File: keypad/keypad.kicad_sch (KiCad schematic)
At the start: 7 parts, among them U1 STM32G031G8Ux

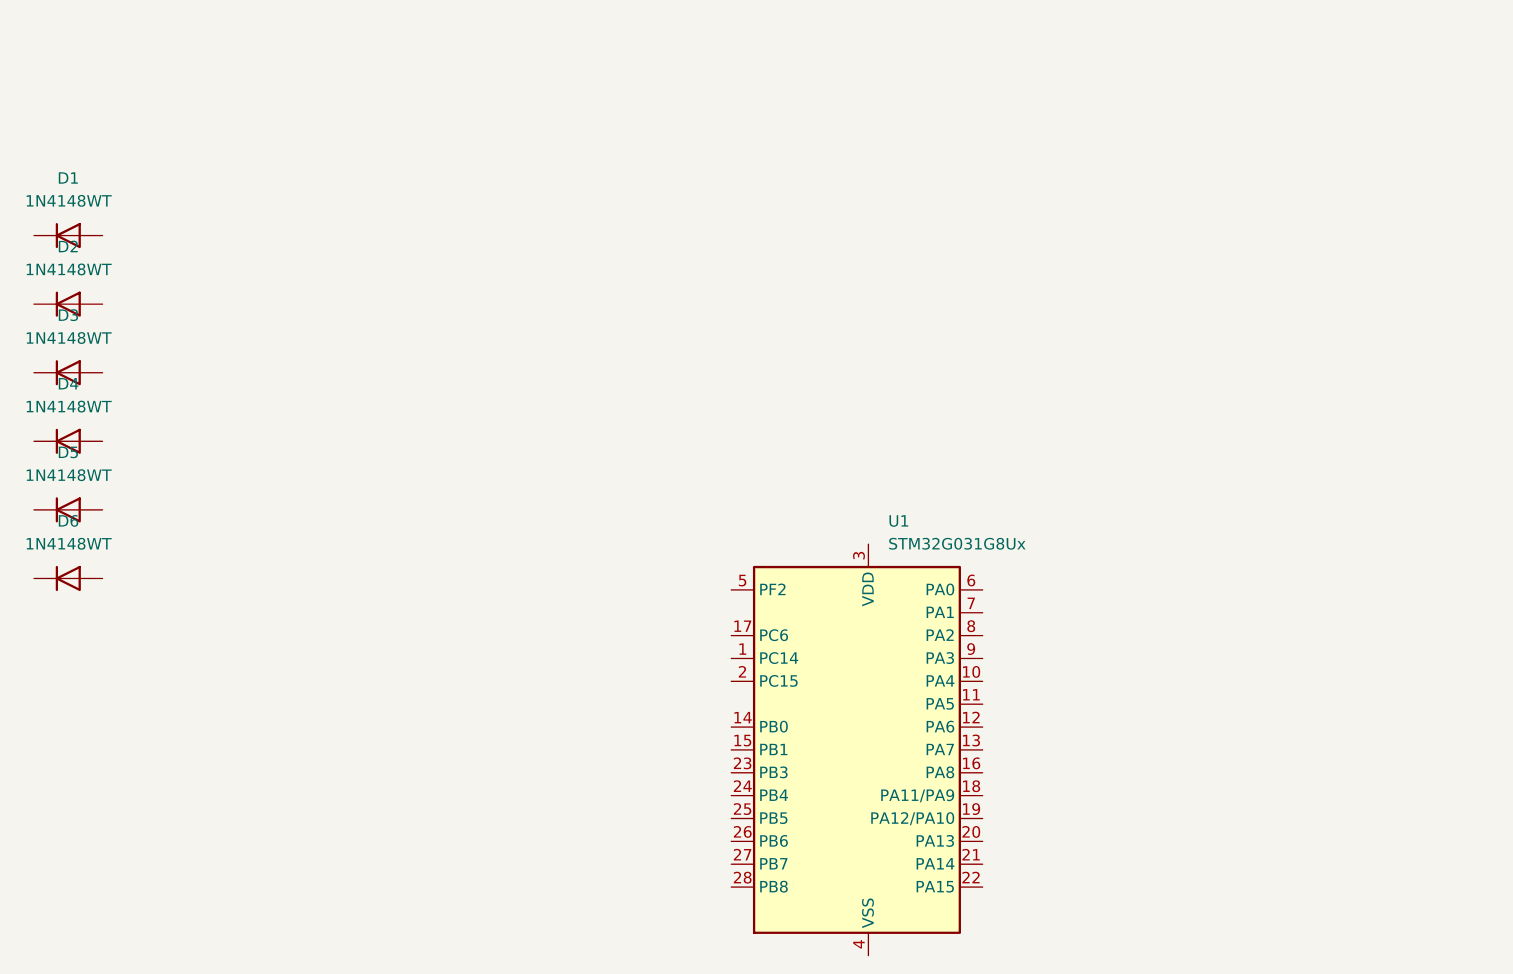
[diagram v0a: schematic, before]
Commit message: main
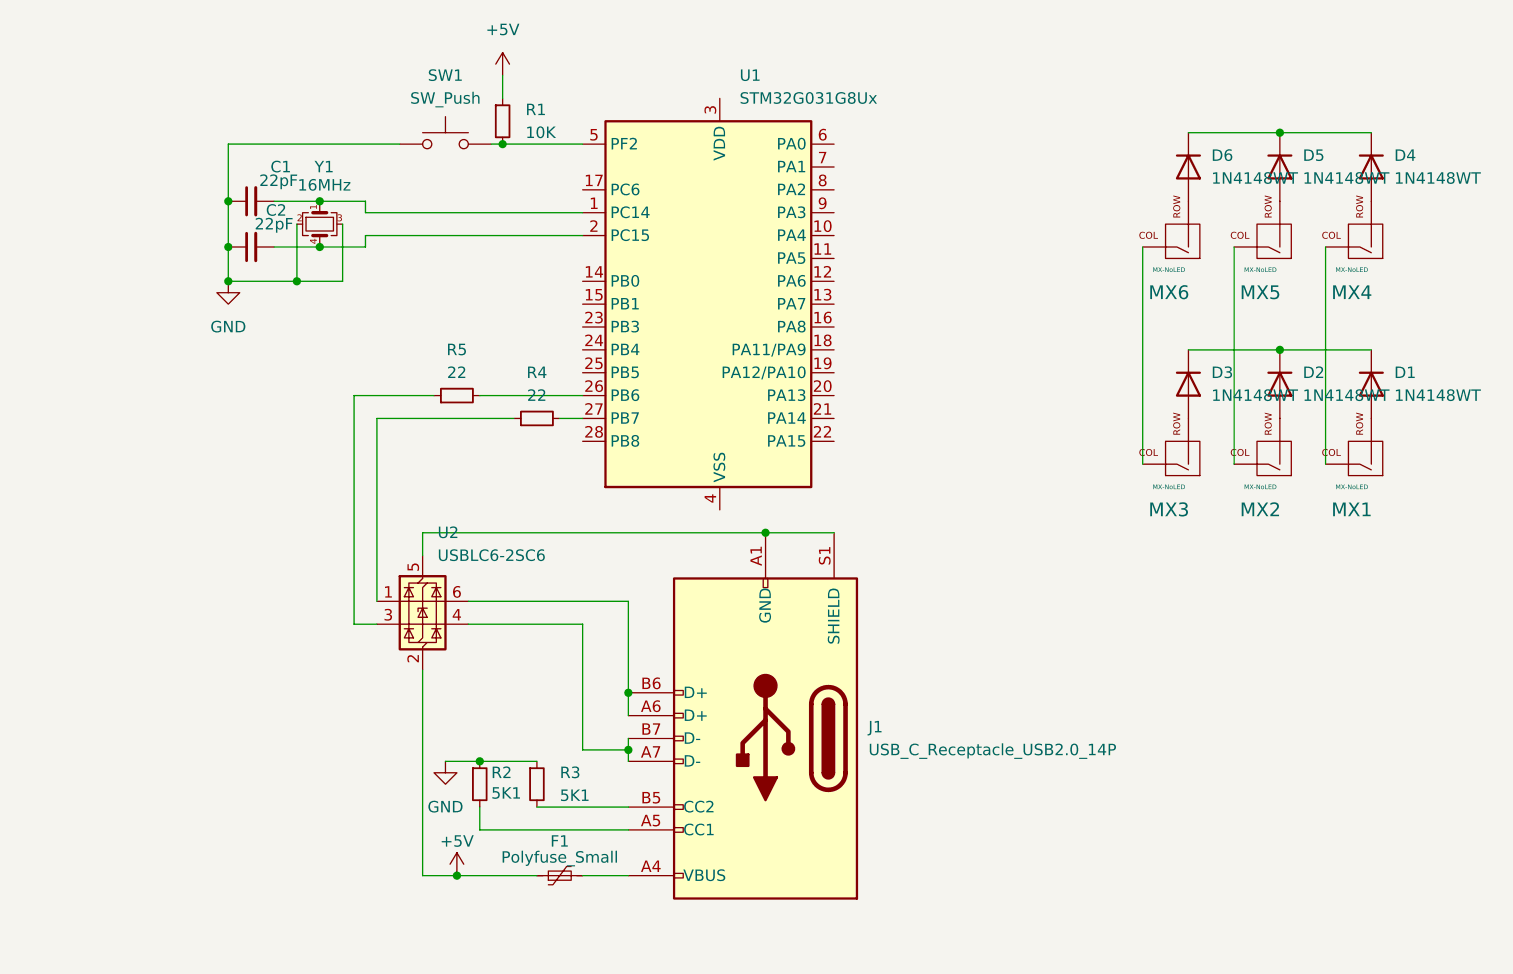
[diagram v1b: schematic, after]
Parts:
- added C1, C2: 22pF, symbol Device:C_Small
- added F1: Polyfuse_Small, symbol Device:Polyfuse_Small
- added J1: USB_C_Receptacle_USB2.0_14P, symbol Connector:USB_C_Receptacle_USB2.0_14P
- added MX1, MX2, MX3, MX4, MX5, MX6: MX-NoLED, symbol MX_Alps_Hybrid:MX-NoLED
- added R1: 10K, symbol Device:R_Small
- added R2, R3: 5K1, symbol Device:R_Small
- added R4, R5: 22, symbol Device:R_Small
- added SW1: SW_Push, symbol Switch:SW_Push
- added U2: USBLC6-2SC6, Package_TO_SOT_SMD:SOT-23-6, symbol Power_Protection:USBLC6-2SC6
- added Y1: 16MHz, symbol Device:Crystal_GND23_Small
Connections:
- net at D3.1 (K): now also D1.1 (K), D2.1 (K)
- net at D3.2 (A): now also MX3.2 (ROW)
- net at U1.1 (PC14): now also C1.2, Y1.1
- net at U1.2 (PC15): now also C2.2, Y1.4
- net at U1.26 (PB6): now also R5.2
- net at U1.27 (PB7): now also R4.2
- net at U1.5 (PF2): now also R1.2, SW1.2
- net at D2.2 (A): now also MX2.2 (ROW)
- net at D6.1 (K): now also D4.1 (K), D5.1 (K)
- net at D6.2 (A): now also MX6.2 (ROW)
- net at D4.2 (A): now also MX4.2 (ROW)
- net at D1.2 (A): now also MX1.2 (ROW)
- net at D5.2 (A): now also MX5.2 (ROW)
- new net: J1.A1 (GND), J1.A12 (GND), J1.B1 (GND), J1.B12 (GND), J1.S1 (SHIELD), U2.5 (VBUS)
- new net: F1.2, J1.A4 (VBUS), J1.A9 (VBUS), J1.B4 (VBUS), J1.B9 (VBUS)
- new net: J1.A5 (CC1), R2.2
- new net: J1.A6 (D+), J1.B6 (D+), U2.6 (I/O1)
- new net: J1.A7 (D-), J1.B7 (D-), U2.4 (I/O2)
- new net: J1.B5 (CC2), R3.2
- new net: MX1.1 (COL), MX4.1 (COL)
- new net: MX2.1 (COL), MX5.1 (COL)
- new net: MX3.1 (COL), MX6.1 (COL)
- new net: R4.1, U2.1 (I/O1)
- new net: R5.1, U2.3 (I/O2)
- new net +5V: F1.1, R1.1, U2.2 (GND)
- new net GND: C1.1, C2.1, R2.1, R3.1, SW1.1, Y1.2, Y1.3
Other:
- moved on the sheet: D1, D2, D3, D4, D5, D6, U1
